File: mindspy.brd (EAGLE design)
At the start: 45.7 x 50.8 mm, 40 parts, among them IC1 ADS1298IPAG, IC2 TPS7A4901, X1 DF9-31S, X2 STELLARIS-LAUNCHPAD-HALF

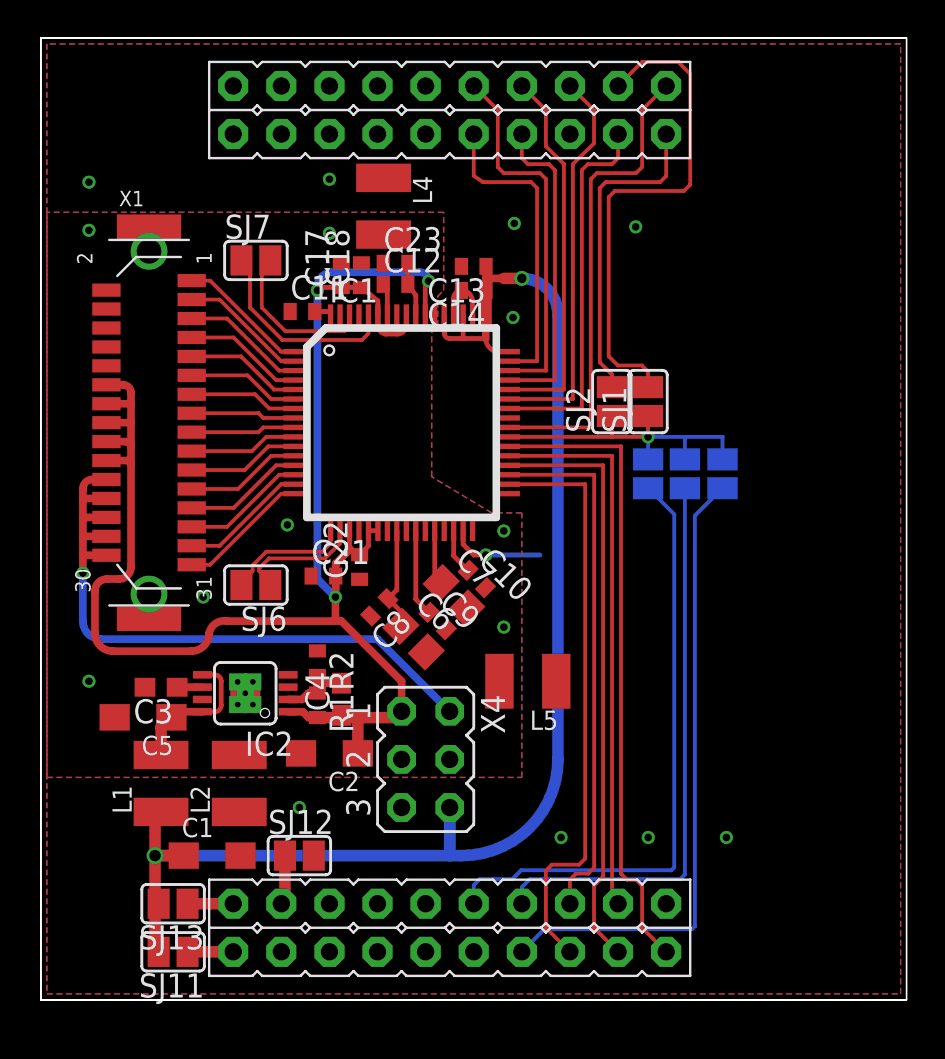
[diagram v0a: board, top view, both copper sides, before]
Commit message: Major changes
* placing improvements
 * labels on board
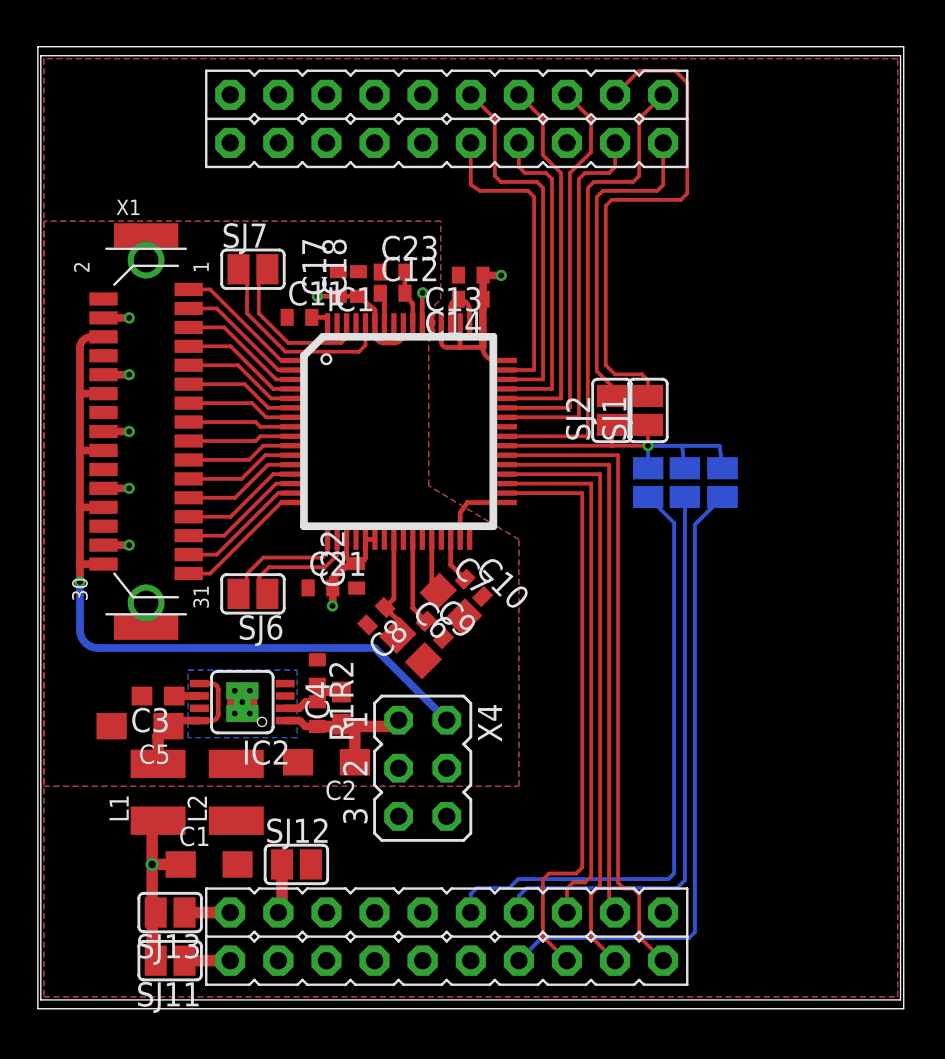
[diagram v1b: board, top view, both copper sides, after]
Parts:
- removed L4, L5: 10u, fabhack:L1210K
- moved C21 0.64 mm to (14.8, 21.8)
- moved C23 0.49 mm to (18.6, 38.4)
- moved C17 0.49 mm to (15.7, 37.8)
- moved SJ7 0.49 mm to (11.2, 38.6)
- moved C14 0.49 mm to (22.7, 37.0)
- moved C18 0.49 mm to (16.8, 37.8)
- moved C22 0.49 mm to (16.7, 22.4)
- moved C7 0.49 mm to (21.7, 20.9)
- moved IC1 0.49 mm to (18.9, 30.0)
- moved C2 0.49 mm to (15.1, 12.6)
- moved SJ12 0.49 mm to (13.5, 7.15)
- moved SJ13 0.49 mm to (6.83, 4.61)
- moved SJ6 0.49 mm to (11.2, 21.4)
- moved C3 0.49 mm to (6.19, 16.0)
- moved C5 0.49 mm to (5.24, 14.5)
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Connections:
- net AVCM: now also X1.12, X1.18, X1.6; no longer X1.22, X1.26, X1.28
- net AVDD: now also X1.10, X1.22, X1.28, X1.4; no longer X1.12, X1.14, X1.18, X1.20
- net AVSS: now also X1.14, X1.20, X1.26; no longer L4.2, L5.2, X1.10, X1.4, X1.6
- net DGND: no longer L4.1, L5.1
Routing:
- net AVDD: track 89.4 -> 30.6 mm, vias 3 -> 8
- net DVDD: track 73.2 -> 20.2 mm
- net AVCM: track 34.8 -> 42.7 mm
- net DGND: track 7.99 -> 7.12 mm, vias 10 -> 0
- net AVSS: vias 7 -> 0
- added copper zone on layer 16, net AVDD
- added copper zone on layer 16, net DVDD
- removed copper zone on layer 16, net DGND
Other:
- board text added: "+"
- board text added: "-"
- board text added: "0V"
- board text added: "100uH"
- board text added: "10k"
- board text added: "10n"
- board text added: "10u"
- board text added: "18u"
- board text added: "1u"
- board text added: "24k"
- board text added: "3V3"
- board text added: "4n7"
- board text added: "5V"
- board text added: "RLDREF/IN"
- board text added: "TESTP/N"
- board text added: "u1"
- board text added: "ver. 0.2"
- board text removed: "RLDIN"
- board text removed: "RLDREF"
- board text removed: "TESTN"
- board text removed: "TESTP"
- board text removed: "ver. 0.1"
